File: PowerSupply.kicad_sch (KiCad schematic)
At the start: 87 parts, among them J14 PROG, J2 39-30-0060, J3 ENABLE, Q10 FDC5614P, Q5 BSC040N08NS5ATMA1, Q6 BSC040N08NS5ATMA1, Q7 2N7002K, Q8 NTD5867NLT4G, Q9 2N7002K, U2 ATtiny1616-S, U4 TSC2012IDT, U6 L7987, U7 AZ1117IH-3.3TRG1, U8 LM74800QDRRRQ1

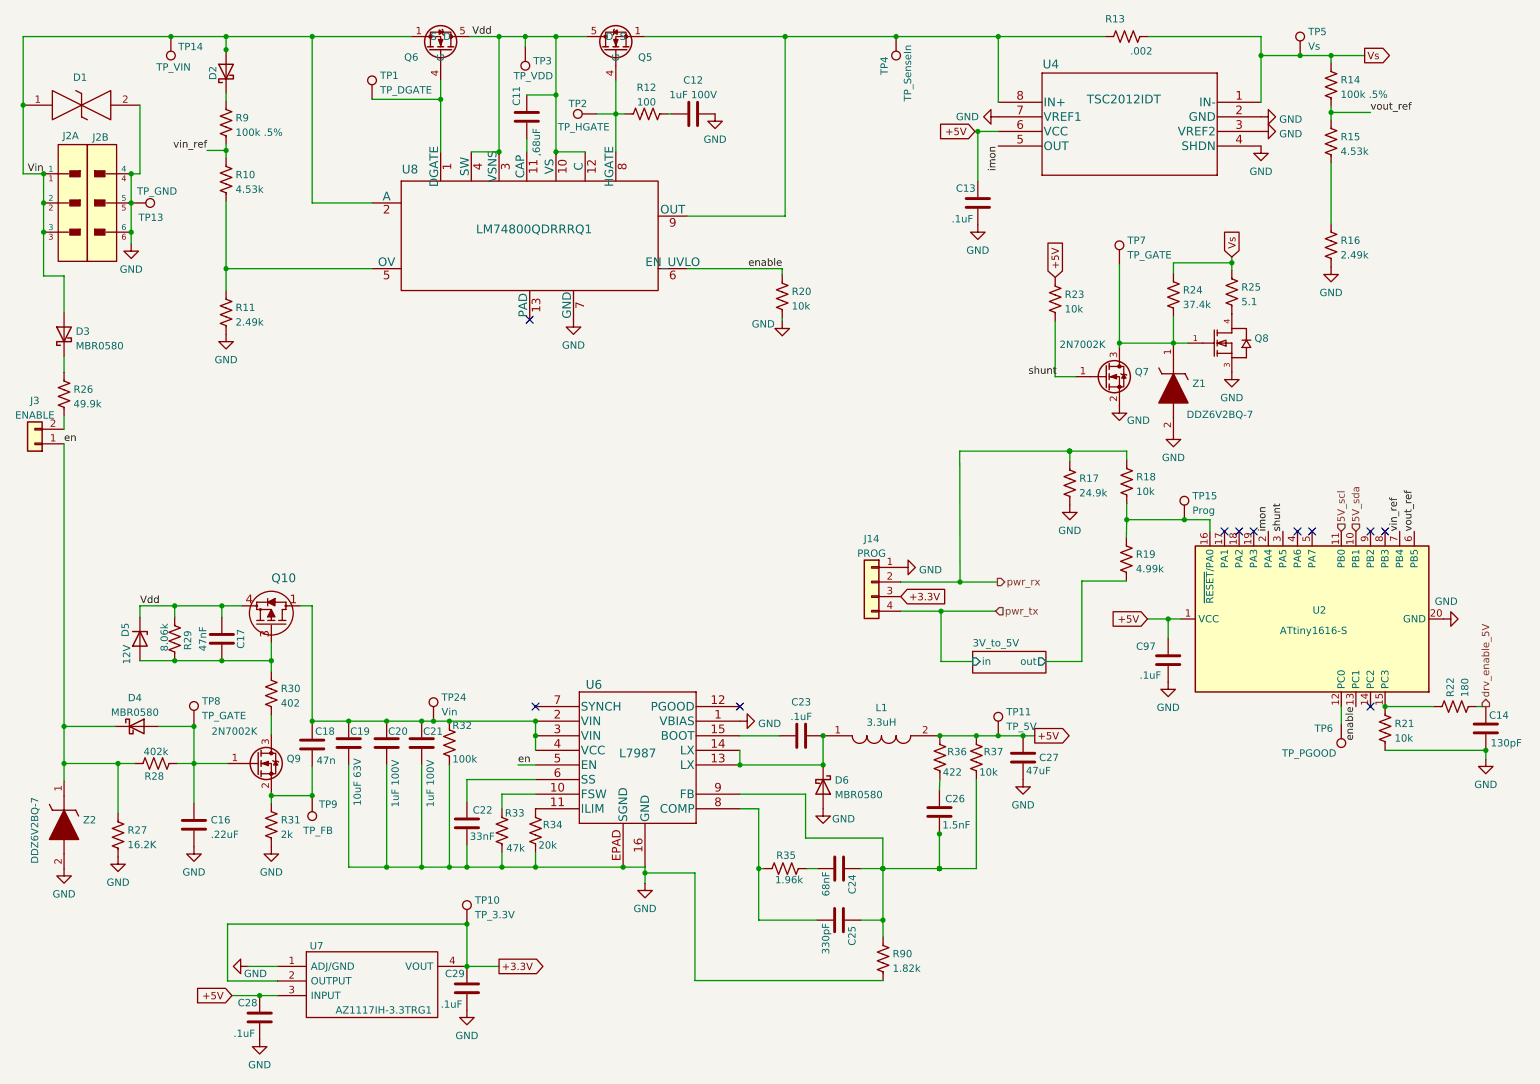
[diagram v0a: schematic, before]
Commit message: put all schematics on 50 mil grid
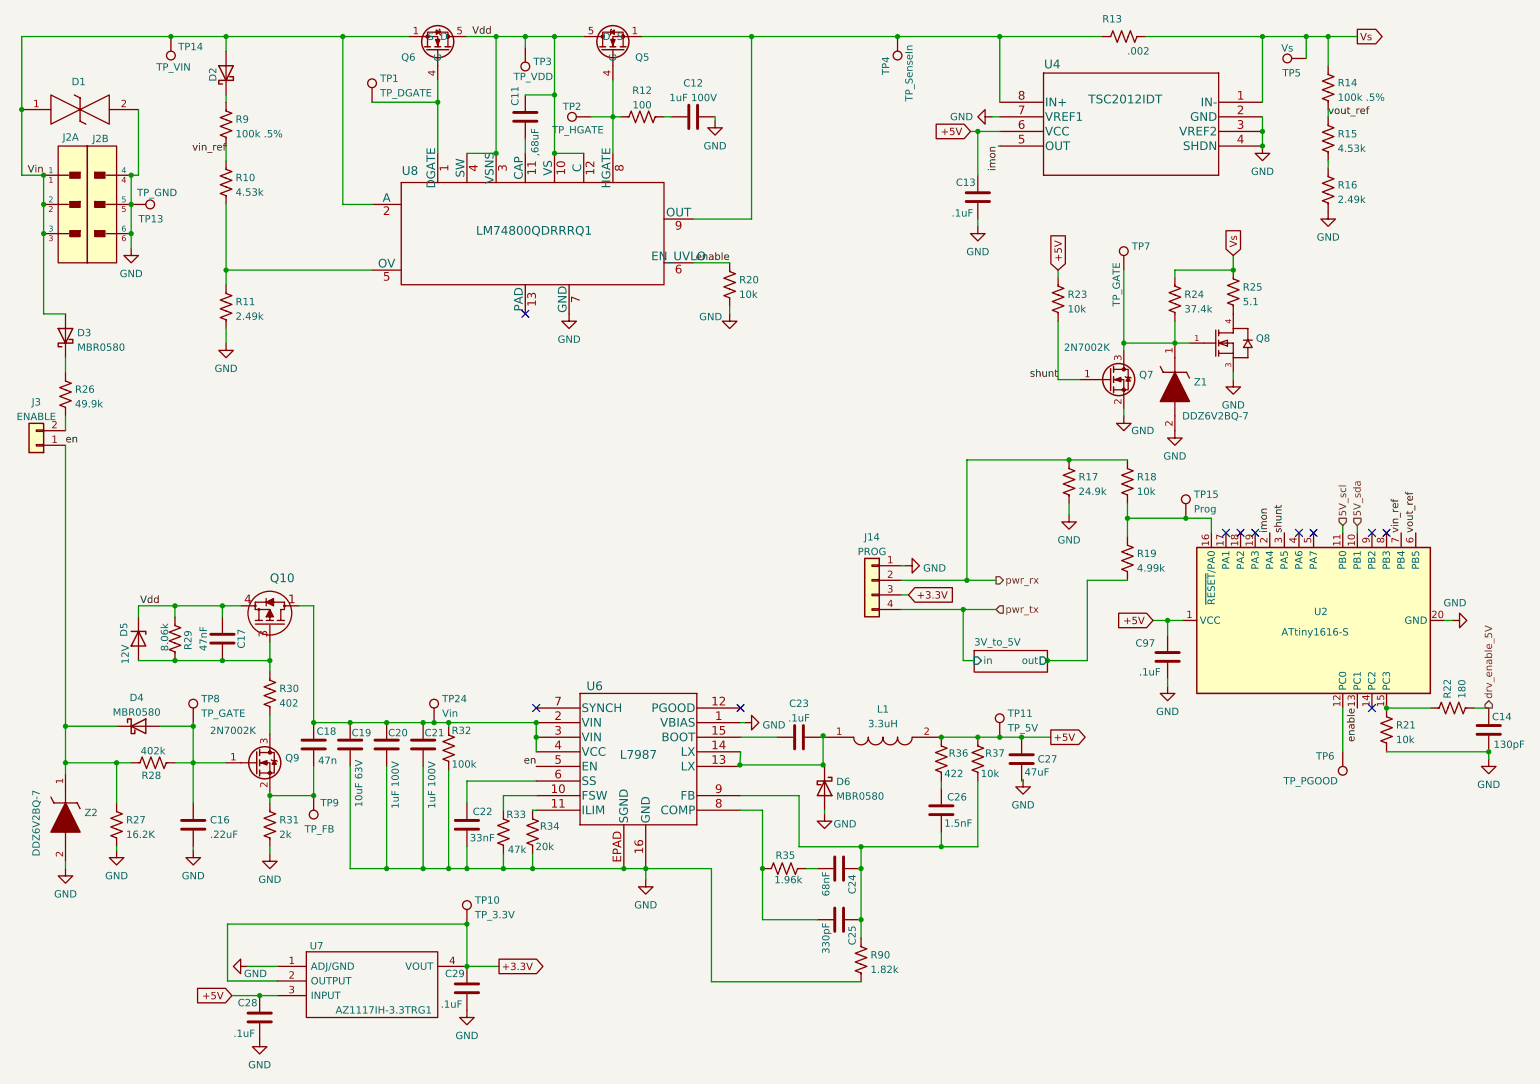
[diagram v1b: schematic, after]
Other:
- moved on the sheet: C12, C13, C14, C97, D1, Q5, Q6, Q7, R10, R11, R12, R13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

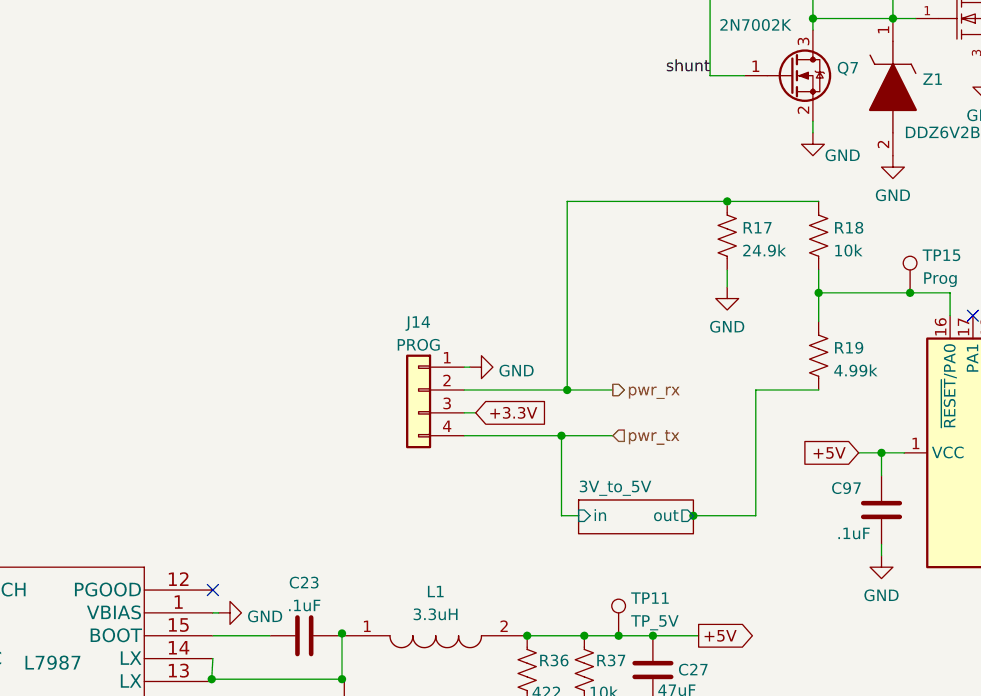
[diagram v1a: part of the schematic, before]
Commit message: first commit of V18
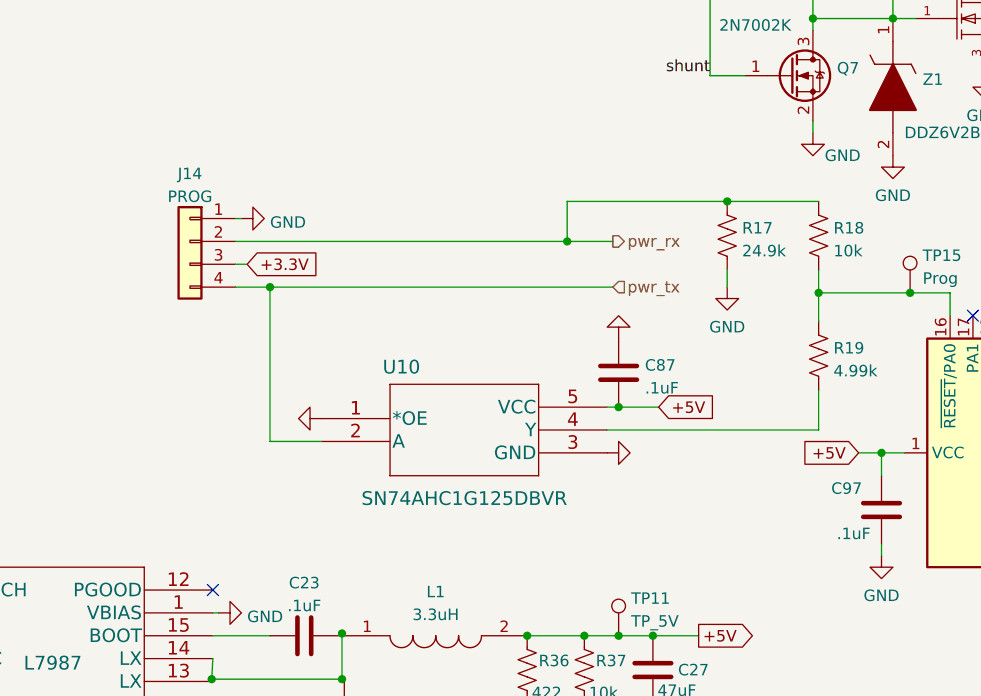
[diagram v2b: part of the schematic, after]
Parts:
- added C87: .1uF, Capacitor_SMD:C_0805_2012Metric_Pad1.18x1.45mm_HandSolder, symbol Device:C
- added U10: SN74AHC1G125DBVR, Project_Footprints_Library:SN74AHC1G125DBVR, symbol 1LibBBCTRL:SN74AHC1G125DBVR
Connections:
- net +5V: now also C87.2, U10.5 (VCC)
- net GND: now also C87.1, U10.1 (*OE), U10.3 (GND)
- net pwr_tx: now also U10.2 (A)
- net 3V_to_5V/out: no longer names the net of R19.2
- net 3V_to_5V/out: now also U10.4 (Y)
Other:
- removed sheet 3V_to_5V
- moved on the sheet: J14

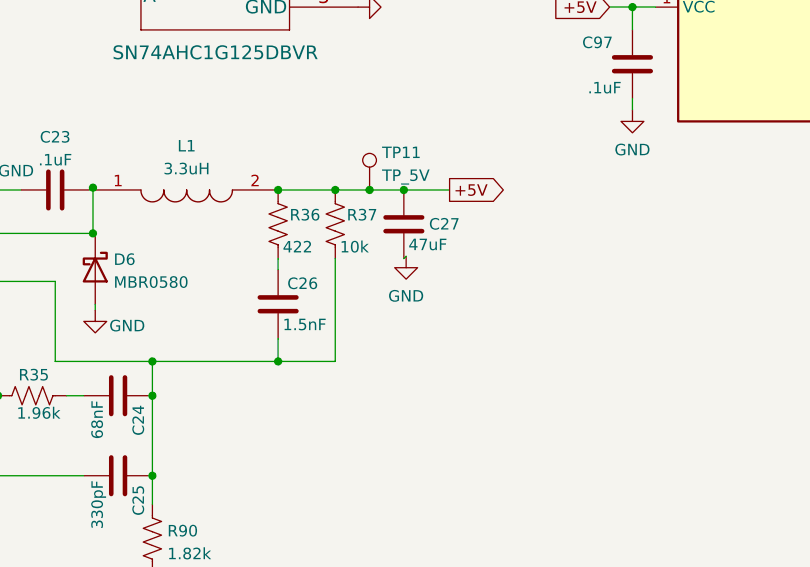
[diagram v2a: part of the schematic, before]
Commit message: added oled support
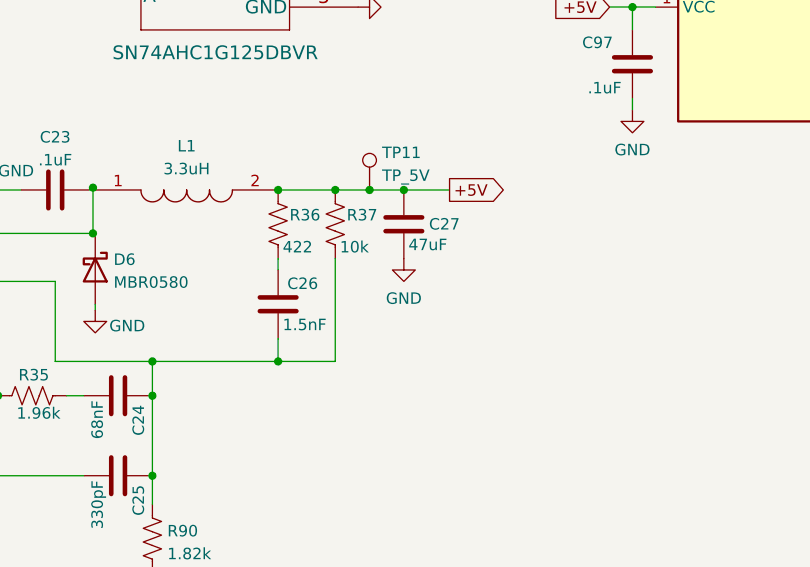
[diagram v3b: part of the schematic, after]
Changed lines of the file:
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@@
-    (stroke (width 0) (type default) (color 0 0 0 0))
-  )
-  (wire (pts (xy 191.77 146.05) (xy 192.024 145.796))
     (stroke (width 0) (type default) (color 0 0 0 0))
   )
@@
     (pin "2")
   )
-  (symbol (lib_id "power:GND") (at 192.024 145.796 0) (unit 1)
-    (in_bom yes) (on_board yes) (fields_autoplaced)
-    (property "Reference" "#PWR0127" (id 0) (at 192.024 152.146 0)
-      (effects (font (size 1.27 1.27)) hide)
-    )
-    (property "Value" "GND" (id 1) (at 192.024 150.2394 0))
-    (property "Footprint" "" (id 2) (at 192.024 145.796 0)
-      (effects (font (size 1.27 1.27)) hide)
-    )
-    (property "Datasheet" "" (id 3) (at 192.024 145.796 0)
-      (effects (font (size 1.27 1.27)) hide)
-    )
+  (symbol (lib_id "power:GND") (at 191.77 146.05 0) (unit 1)
+    (in_bom yes) (on_board yes) (fields_autoplaced)
+    (property "Reference" "#PWR0127" (id 0) (at 191.77 152.4 0)
+      (effects (font (size 1.27 1.27)) hide)
+    )
+    (property "Value" "GND" (id 1) (at 191.77 150.4934 0))
+    (property "Footprint" "" (id 2) (at 191.77 146.05 0)
+      (effects (font (size 1.27 1.27)) hide)
+    )
+    (property "Datasheet" "" (id 3) (at 191.77 146.05 0)
+      (effects (font (size 1.27 1.27)) hide)
+    )
